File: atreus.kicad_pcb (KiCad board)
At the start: 2 copper layers, 232 x 90 mm, 103 parts, among them U1 ATmega32U4-AU, Y1 Crystal_GND24_Small

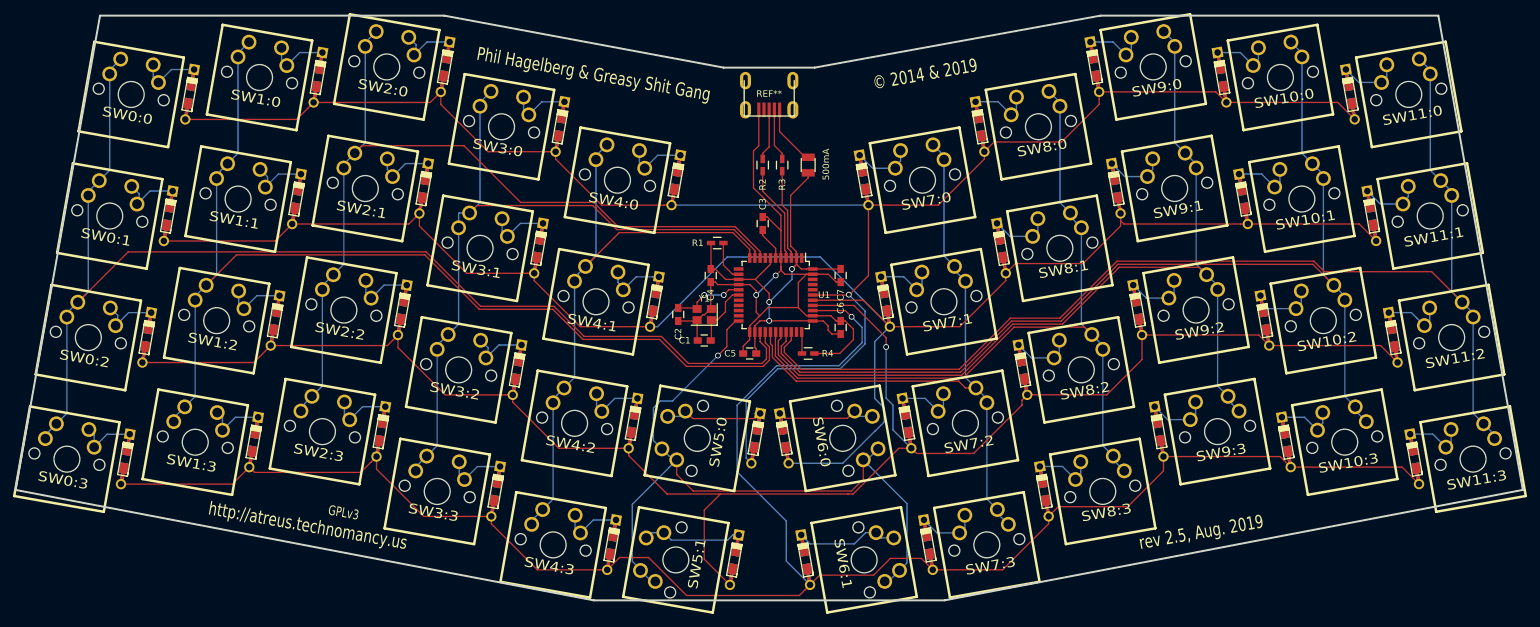
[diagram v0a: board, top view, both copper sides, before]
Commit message: added csv.
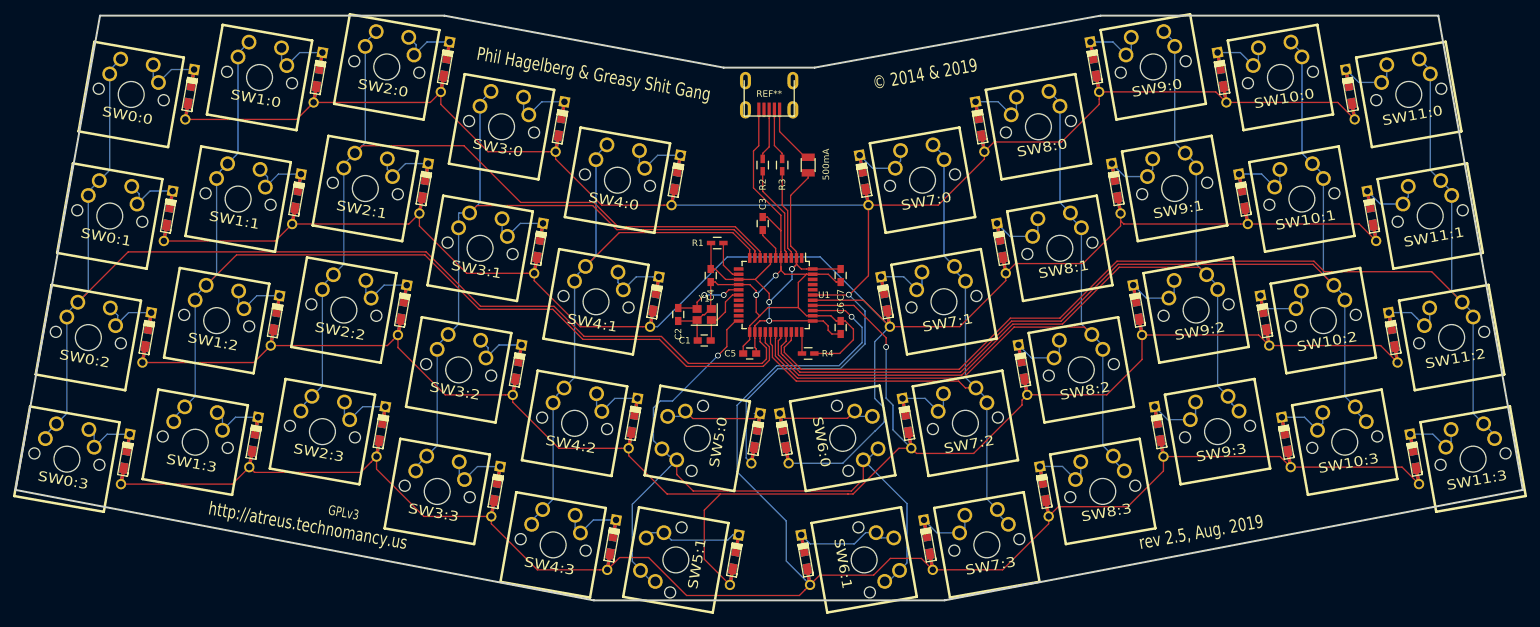
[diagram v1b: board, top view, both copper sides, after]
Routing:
- net GND: track 109.1 -> 0.00 mm, vias 2 -> 0
- net N-diode-45: track 9.37 -> 109.1 mm, vias 0 -> 2
- net 64: track 0.00 -> 73.3 mm, vias 0 -> 3
- net +5V: track 73.3 -> 0.00 mm, vias 3 -> 0
- net N-diode-22: track 0.00 -> 16.4 mm
- net N-diode-23: track 0.00 -> 15.9 mm
- net Net-R2-Pad1: track 14.8 -> 0.00 mm
- net 67: track 0.00 -> 14.8 mm
- net Net-R3-Pad1: track 13.9 -> 0.00 mm
- net 70: track 0.00 -> 13.9 mm
- net Net-C2-Pad1: track 11.2 -> 0.00 mm, vias 2 -> 0
- net Net-C1-Pad1: track 9.87 -> 0.00 mm
- net VCC: track 9.38 -> 0.00 mm
- net 65: track 0.00 -> 9.38 mm
- net N-diode-26: track 0.00 -> 9.37 mm
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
